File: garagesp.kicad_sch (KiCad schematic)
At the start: 29 parts, among them J1 USB_C_Receptacle_USB2.0_14P, J2 AHT21, J3 DOOR CTL, J4 DOOR SW, K1 SANYOU_SRD_Form_A, Q1 BC547, SW1 RESET, SW2 BOOT, U1 ESP32-C3-WROOM-02, U2 AP2112K-3.3

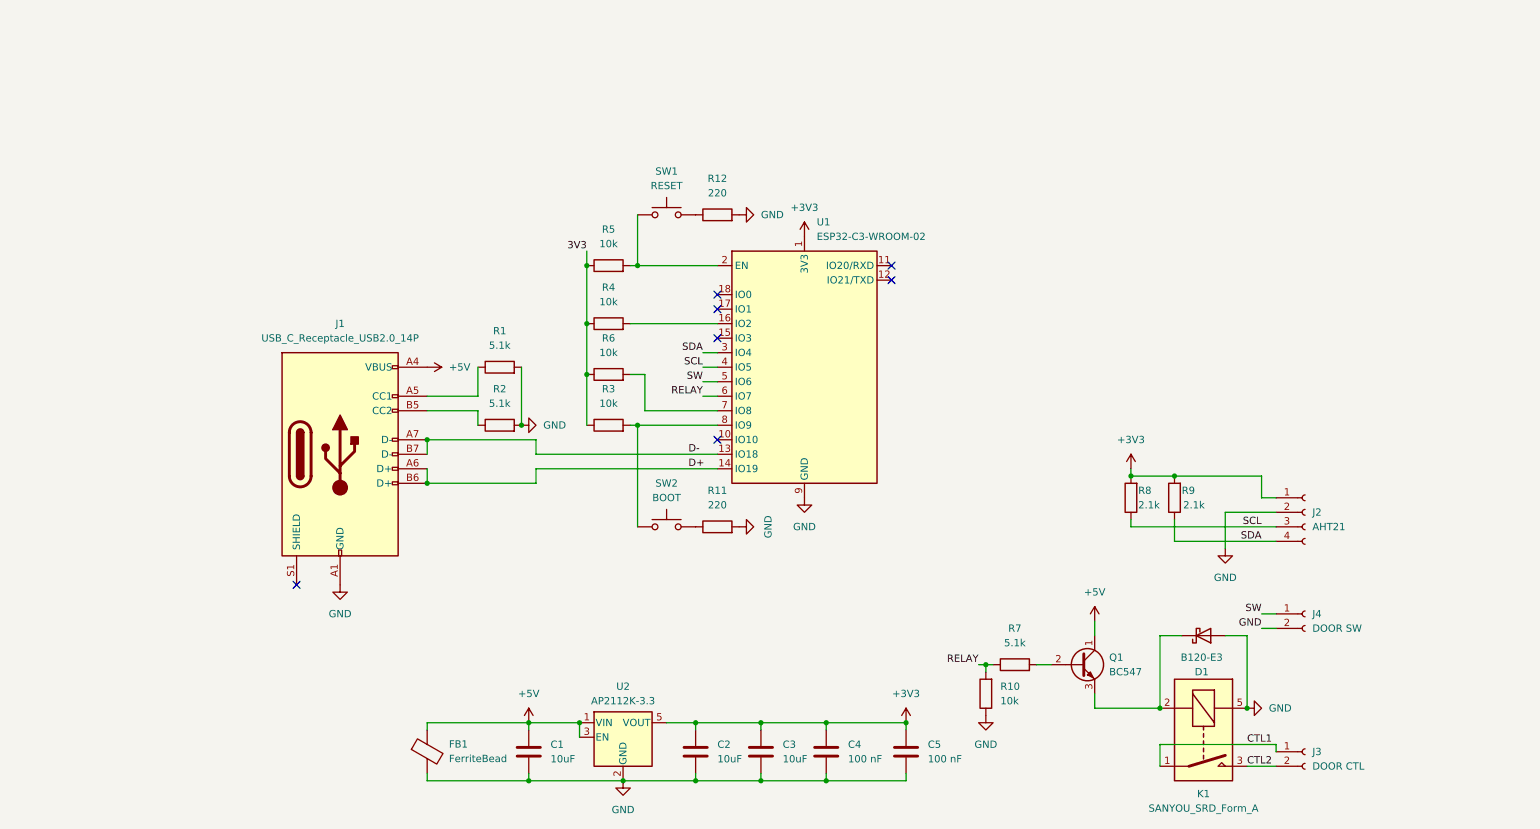
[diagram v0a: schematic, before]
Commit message: add capacitors and resistors
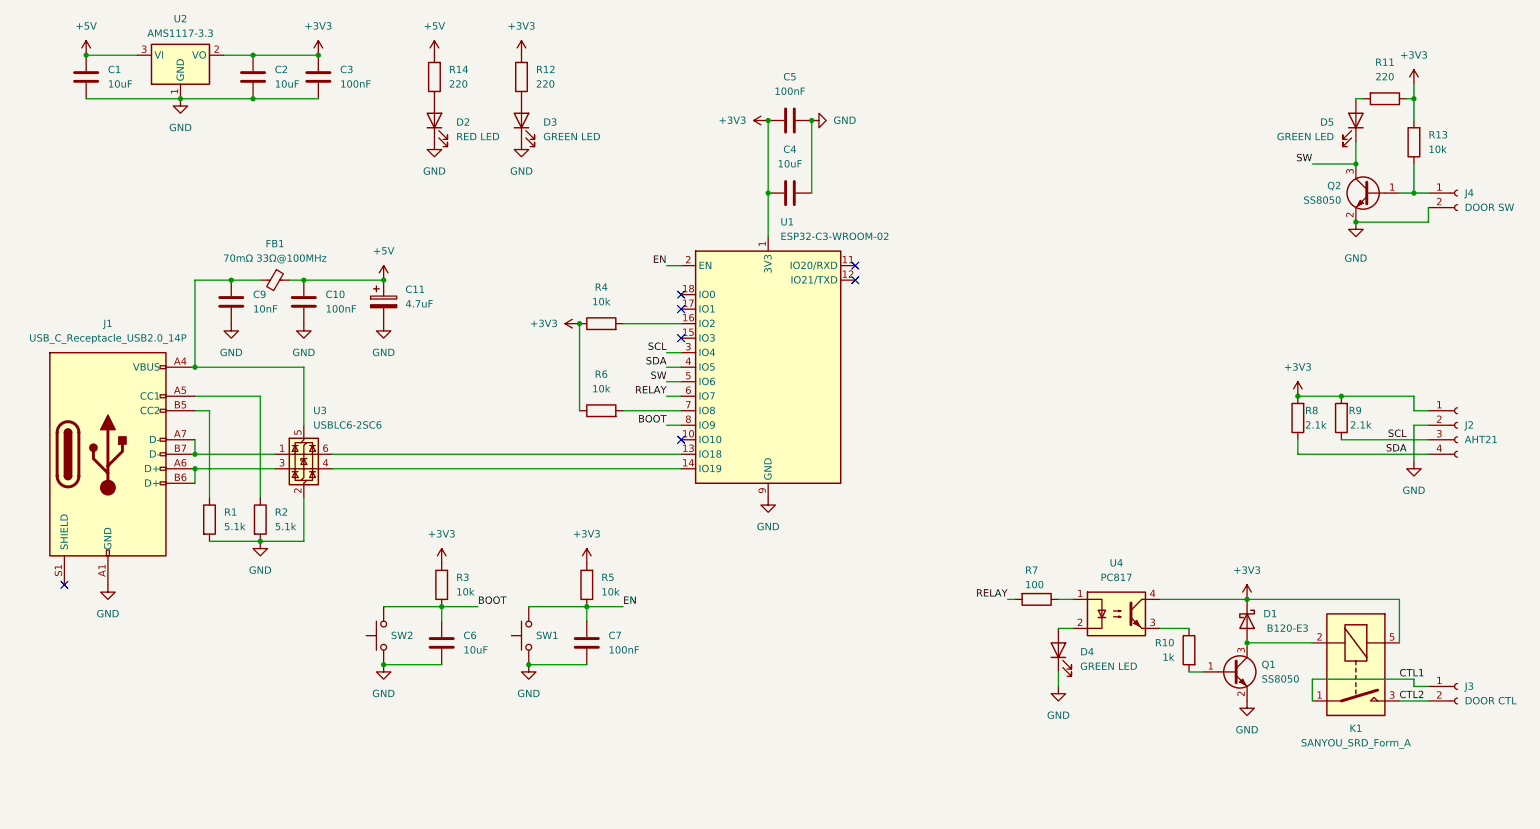
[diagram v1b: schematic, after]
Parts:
- removed C3: 10uF, Capacitor_SMD:C_0805_2012Metric_Pad1.18x1.45mm_HandSolder, symbol Device:C
- removed Q1: BC547, Package_TO_SOT_THT:TO-92_Inline, symbol Transistor_BJT:BC547
- removed U2: AP2112K-3.3, Package_TO_SOT_SMD:SOT-23-5, symbol Regulator_Linear:AP2112K-3.3
- added C10, C7: 100nF, Capacitor_SMD:C_0805_2012Metric_Pad1.18x1.45mm_HandSolder, symbol Device:C
- added C11: 4.7uF, symbol Device:C_Polarized
- added C4, C6: 10uF, Capacitor_SMD:C_0805_2012Metric_Pad1.18x1.45mm_HandSolder, symbol Device:C
- added C9: 10nF, Capacitor_SMD:C_0603_1608Metric_Pad1.08x0.95mm_HandSolder, symbol Device:C
- added D2: RED LED, LED_SMD:LED_0603_1608Metric_Pad1.05x0.95mm_HandSolder, symbol Device:LED
- added D3, D4, D5: GREEN LED, LED_SMD:LED_0603_1608Metric_Pad1.05x0.95mm_HandSolder, symbol Device:LED
- added Q1, Q2: SS8050, Package_TO_SOT_SMD:SOT-23, symbol Transistor_BJT:SS8050
- added R13: 10k, Resistor_SMD:R_0805_2012Metric_Pad1.20x1.40mm_HandSolder, symbol Device:R
- added R14: 220, Resistor_SMD:R_0805_2012Metric_Pad1.20x1.40mm_HandSolder, symbol Device:R
- added U2: AMS1117-3.3, Package_TO_SOT_SMD:SOT-223-3_TabPin2, symbol Regulator_Linear:AMS1117-3.3
- added U3: USBLC6-2SC6, Package_TO_SOT_SMD:SOT-23-6, symbol Power_Protection:USBLC6-2SC6
- added U4: PC817, Package_DIP:DIP-4_W7.62mm, symbol Isolator:PC817
- C3: renamed from C4; value 100 nF -> 100nF
- C5: value 100 nF -> 100nF
- FB1: value FerriteBead -> 70mΩ 33Ω@100MHz; footprint (none) -> Inductor_SMD:L_0805_2012Metric_Pad1.05x1.20mm_HandSolder; symbol Device:FerriteBead -> Device:FerriteBead_Small; LCSC (none) -> C74764
- R10: value 10k -> 1k; LCSC C17414 -> (none)
- R7: value 5.1k -> 100; LCSC C27834 -> (none)
- SW1: value RESET -> ~
- SW2: value BOOT -> ~
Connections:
- net +3V3: now also D1.1 (K), K1.5, R11.1, R12.2, R3.2, R4.1, R5.2, R6.1, C4.1, R13.2, U2.2 (VO), U4.4
- net +5V: now also C10.1, C11.1, R14.2, U2.3 (VI); no longer J1.A4 (VBUS), J1.A9 (VBUS), J1.B4 (VBUS), J1.B9 (VBUS)
- net GND: now also SW1.1, SW2.1, C10.2, C11.2, C4.2, C6.2, C7.1, C9.2, D2.1 (K), D3.1 (K), D4.1 (K), Q1.2 (E), Q2.2 (E), U2.1 (GND), U3.2 (GND); no longer D1.2 (A), FB1.2, K1.5, R10.1, R11.2, R12.2
- net RELAY: now also R7.2; no longer R10.2, R7.1
- net SCL: now also R9.1, U1.3 (IO4); no longer R8.1, U1.4 (IO5)
- net SDA: now also R8.1, U1.4 (IO5); no longer R9.1, U1.3 (IO4)
- net SW: now also D5.1 (K), Q2.3 (C); no longer J4.1 (Pin_1)
- net at R12.1: now also D3.2 (A); no longer SW1.2
- net at R2.1: now also J1.A5 (CC1); no longer J1.B5 (CC2)
- net at K1.2: now also D1.2 (A), Q1.3 (C); no longer D1.1 (K)
- net at R1.1: now also J1.B5 (CC2); no longer J1.A5 (CC1)
- net BOOT: now reaches SW2.2
- net BOOT: now also R3.1, U1.8 (IO9), C6.1; no longer R11.1
- removed net 3V3: R3.1, R4.1, R5.1, R6.1
- net D+: no longer names the net of J1.A6 (D+), J1.B6 (D+)
- net D+: now also U3.3 (I/O2); no longer U1.14 (IO19)
- net D-: no longer names the net of J1.A7 (D-), J1.B7 (D-)
- net D-: now also U3.1 (I/O1); no longer U1.13 (IO18)
- new net: J4.1 (Pin_1), Q2.1 (B), R13.1
- new net: R7.1, U4.1
- new net: D5.2 (A), R11.2
- new net: Q1.1 (B), R10.2
- new net: D2.2 (A), R14.1
- new net: C9.1, FB1.2, J1.A4 (VBUS), J1.A9 (VBUS), J1.B4 (VBUS), J1.B9 (VBUS), U3.5 (VBUS)
- new net: D4.2 (A), U4.2
- new net: U1.14 (IO19), U3.4 (I/O2)
- new net: U1.13 (IO18), U3.6 (I/O1)
- new net: R10.1, U4.3
- new net EN: C7.2, R5.1, SW1.2, U1.2 (EN)
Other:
- moved on the sheet: C1, C2, C3, D1, FB1, J1, J2, J3, J4, K1, R1, R10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
